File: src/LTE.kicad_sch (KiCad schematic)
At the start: 61 parts, among them J11 Conn_IPEX, J9 SIM_NANO_Socket, Q18 SI2308A, Q7 BC817-40-7-F, Q8 BC817-40-7-F, U15 TXS0104ERGYR, U16 LE910R1

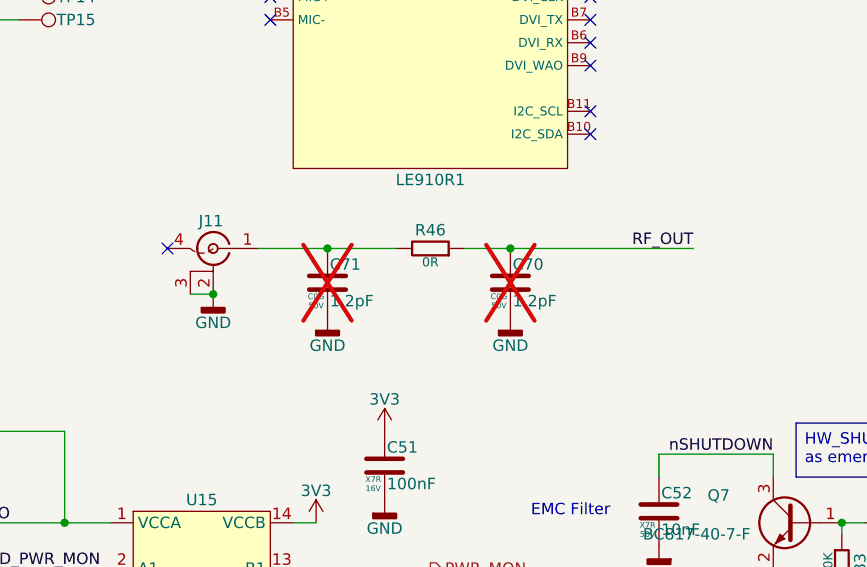
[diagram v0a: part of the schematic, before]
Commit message: layout continued
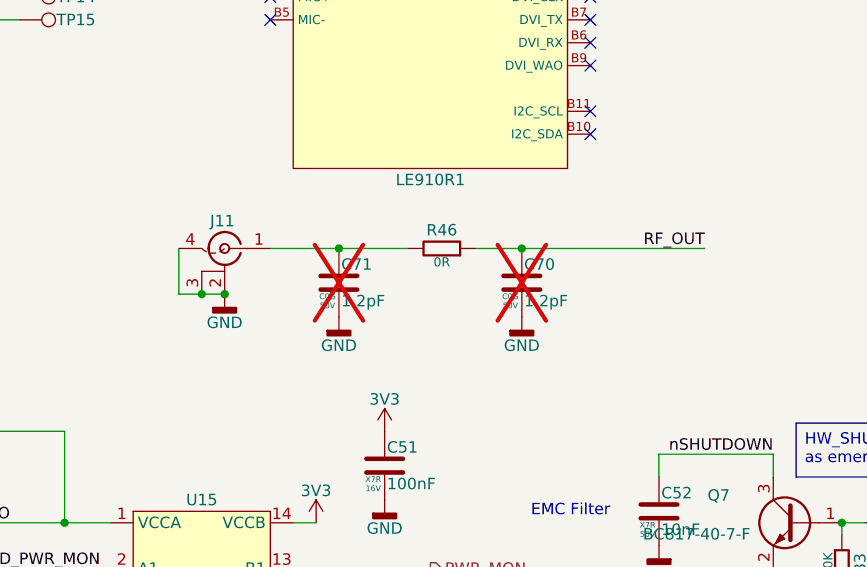
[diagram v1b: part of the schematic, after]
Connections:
- net GND: now also J11.4 (PT)
- no-connect marks 40 -> 39
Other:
- moved on the sheet: C70, C71, J11, R46
